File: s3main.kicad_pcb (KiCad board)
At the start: 2 copper layers, 75 x 60 mm, 142 parts, among them J1 TRACK, J2 IDC, J3 POWER, J4 USB_C_Receptacle_USB2.0_16P, J5 ZUSI, Q1 QS6K21, Q2 BC847BDW1, Q3 SiS4634LDN, Q4 SiS4634LDN, Q5 SiS4634LDN, Q6 QS6K21, Q7 SiS4634LDN, Q8 SiS4634LDN, Q9 BC847B, SW1 EN, SW2 BOOT, U1 LM393, U10 BTS4141N, U2 7402, U3 TLV9061xDBV, U4 ESP32-S3-WROOM-2, U5 DRV8328B, U6 TPS281C100A, U7 AP63205WU, U8 TXS0102DCT, U9 AZ1117-3.3

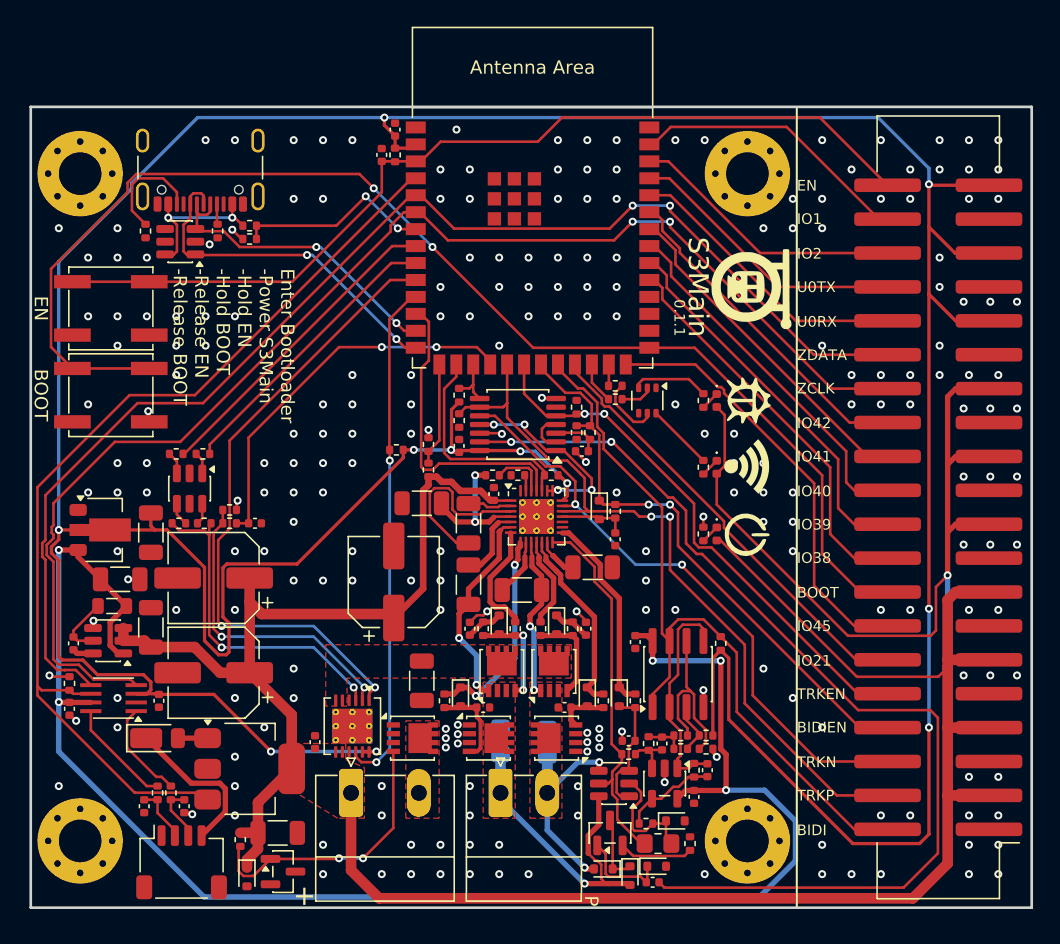
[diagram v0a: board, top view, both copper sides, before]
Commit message: revert: chore: replace ACK circuit with TPS281C100 fault pin
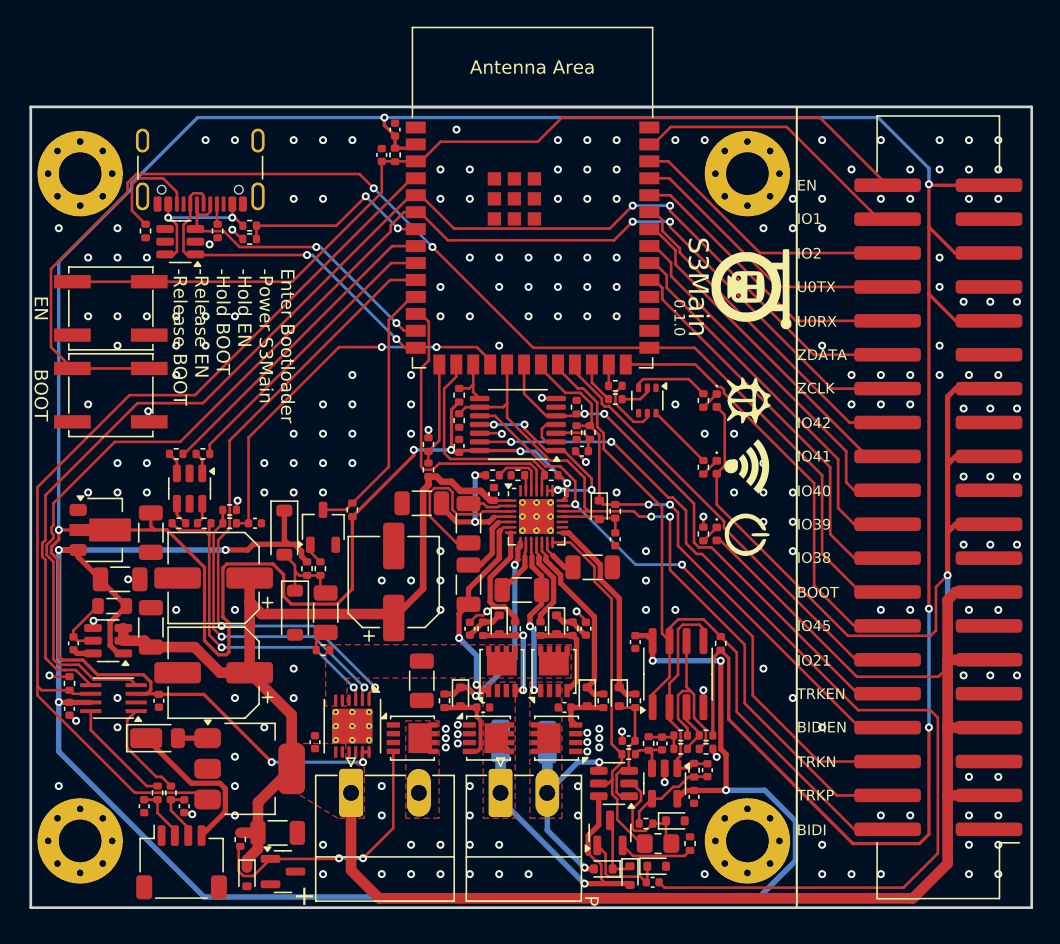
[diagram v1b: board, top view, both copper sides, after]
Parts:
- added C31: 10n, Capacitor_SMD:C_1206_3216Metric, F.Cu at (137.6, 105.4)
- added D14: B5819W, Diode_SMD:D_SOD-123, F.Cu at (134.5, 99.4)
- added D15: B5819W, Diode_SMD:D_SOD-123, F.Cu at (135.3, 105.4)
- added Q9: BSS138, Package_TO_SOT_SMD:TSOT-23, F.Cu at (137.4, 99.0)
- added R49: 4k7, Resistor_SMD:R_0402_1005Metric, F.Cu at (137.4, 108.2)
- added R50: 10k, Resistor_SMD:R_0402_1005Metric, F.Cu at (136.2, 102.1)
- added R51: 1k, Resistor_SMD:R_0402_1005Metric, F.Cu at (137.2, 102.1)
- moved R54 5.58 mm to (139.6, 97.7), turned to 90 degrees
- renumbered C31 to C32, C32 to C33, C33 to C34, C34 to C35, C35 to C36, C36 to C37, D14 to D16, D15 to D17, D16 to D18, D17 to D19, Q9 to Q10, R35 to R34, R36 to R35, R37 to R36, R38 to R37, R39 to R38, R40 to R39, R41 to R40, R42 to R41, R43 to R42, R44 to R43, R45 to R44, R46 to R45, R47 to R46, R48 to R47, R49 to R48, R50 to R52, R51 to R53, R34 to R54, R52 to R55
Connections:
- U6 pad 10: ACK -> unconnected-(U6-~{FAULT}-Pad10)
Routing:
- net +5V: track 214.3 -> 236.5 mm, vias 6 -> 7
- net ACK: track 38.7 -> 20.4 mm, vias 2 -> 0
- net Net-(D14-A): track 0.00 -> 6.54 mm
- net +3V3: track 297.5 -> 303.5 mm
- net Net-(C31-Pad1): track 0.00 -> 1.62 mm
- net Net-(Q9-G): track 0.00 -> 1.59 mm
- net GND: vias 238 -> 231
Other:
- board text added: "0.1.0"
- board text removed: "0.1.1"

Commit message: chore: replace ACK circuit with TPS281C100 fault pin
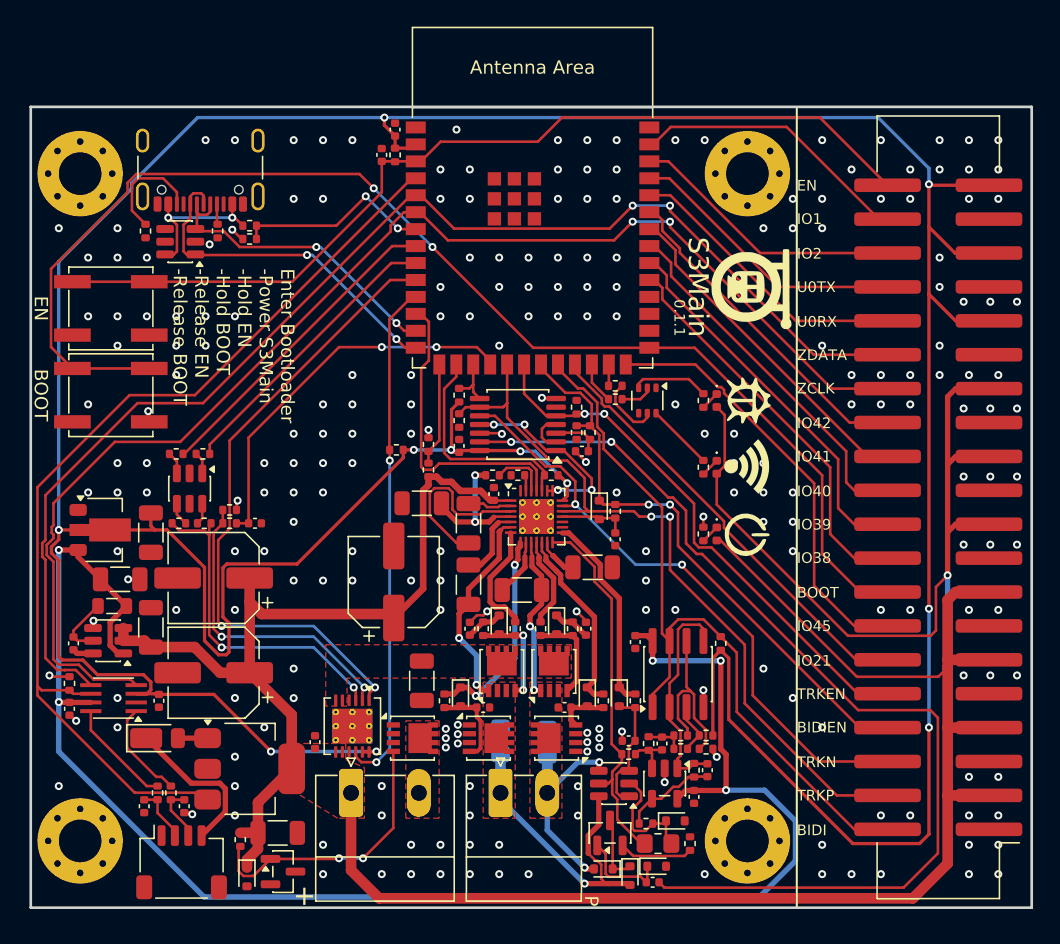
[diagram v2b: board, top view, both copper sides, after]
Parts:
- removed the C31 at (137.6, 105.4)
- removed the D14 at (134.5, 99.4)
- removed the D15 at (135.3, 105.4)
- removed the Q9 at (137.4, 99.0)
- removed the R49 at (137.4, 108.2)
- removed the R50 at (136.2, 102.1)
- removed the R51 at (137.2, 102.1)
- moved R34 5.58 mm to (142.9, 93.2), turned to 180 degrees
- renumbered C32 to C31, C33 to C32, C34 to C33, C35 to C34, C36 to C35, C37 to C36, D16 to D14, D17 to D15, D18 to D16, D19 to D17, Q10 to Q9, R54 to R34, R34 to R35, R35 to R36, R36 to R37, R37 to R38, R38 to R39, R39 to R40, R40 to R41, R41 to R42, R42 to R43, R43 to R44, R44 to R45, R45 to R46, R46 to R47, R47 to R48, R48 to R49, R52 to R50, R53 to R51, R55 to R52
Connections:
- U6 pad 10: unconnected-(U6-~{FAULT}-Pad10) -> ACK
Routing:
- net +5V: track 236.5 -> 214.3 mm, vias 7 -> 6
- net ACK: track 20.4 -> 38.7 mm, vias 0 -> 2
- net Net-(D14-A): track 6.54 -> 0.00 mm
- net +3V3: track 303.5 -> 297.5 mm
- net Net-(C31-Pad1): track 1.62 -> 0.00 mm
- net Net-(Q9-G): track 1.59 -> 0.00 mm
- net GND: vias 231 -> 238
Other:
- board text added: "0.1.1"
- board text removed: "0.1.0"
